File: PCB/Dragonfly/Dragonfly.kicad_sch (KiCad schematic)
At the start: 0 parts

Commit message: hell yeah
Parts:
- added U1: STM32F405RGTx, Package_QFP:LQFP-64_10x10mm_P0.5mm, symbol MCU_ST_STM32F4:STM32F405RGTx
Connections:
- new net: U1.18 (VSS), U1.63 (VSS)
- new net PA0: U1.14 (PA0)
- new net PA1: U1.15 (PA1)
- new net PA10: U1.43 (PA10)
- new net PA11: U1.44 (PA11)
- new net PA12: U1.45 (PA12)
- new net PA13: U1.46 (PA13)
- new net PA14: U1.49 (PA14)
- new net PA15: U1.50 (PA15)
- new net PA2: U1.16 (PA2)
- new net PA3: U1.17 (PA3)
- new net PA4: U1.20 (PA4)
- new net PA5: U1.21 (PA5)
- new net PA6: U1.22 (PA6)
- new net PA7: U1.23 (PA7)
- new net PA8: U1.41 (PA8)
- new net PA9: U1.42 (PA9)
- new net PB0: U1.26 (PB0)
- new net PB1: U1.27 (PB1)
- new net PB10: U1.29 (PB10)
- new net PB11: U1.30 (PB11)
- new net PB12: U1.33 (PB12)
- new net PB13: U1.34 (PB13)
- new net PB14: U1.35 (PB14)
- new net PB15: U1.36 (PB15)
- new net PB2: U1.28 (PB2)
- new net PB3: U1.55 (PB3)
- new net PB4: U1.56 (PB4)
- new net PB5: U1.57 (PB5)
- new net PB6: U1.58 (PB6)
- new net PB7: U1.59 (PB7)
- new net PB8: U1.61 (PB8)
- new net PB9: U1.62 (PB9)
- new net PC0: U1.8 (PC0)
- new net PC1: U1.9 (PC1)
- new net PC10: U1.51 (PC10)
- new net PC11: U1.52 (PC11)
- new net PC12: U1.53 (PC12)
- new net PC13: U1.2 (PC13)
- new net PC14: U1.3 (PC14)
- new net PC15: U1.4 (PC15)
- new net PC2: U1.10 (PC2)
- new net PC3: U1.11 (PC3)
- new net PC4: U1.24 (PC4)
- new net PC5: U1.25 (PC5)
- new net PC6: U1.37 (PC6)
- new net PC8: U1.38 (PC7)
- new net PC9: U1.39 (PC8)

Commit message: updated
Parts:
- added +10ppm: 32.768 kHz, symbol Device:Crystal
- added C1, C2: 100pf, symbol Device:C
- added C3, C4: 12pf, symbol Device:C
- added SW1: SW_SPDT_312, symbol Switch:SW_SPDT_312
- added X1: TSX-3225, TSX-3225, symbol TSX-3225:TSX-3225
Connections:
- net PC9 is gone; now on net PC8: U1.39 (PC8)
- net PC8: no longer U1.38 (PC7)
- net CP9: now reaches U1.40 (PC9)
- net at U1.5 (PH0): now also C1.2, X1.1
- net PD2: now reaches U1.54 (PD2)
- net at U1.6 (PH1): now also C2.2, X1.3
- net BOOT0: now reaches U1.60 (BOOT0)
- net NRST: now reaches U1.7 (NRST)
- net PA14: no longer names the net of U1.49 (PA14)
- net PA14: now also +10ppm.2, C3.1
- net PA15: no longer names the net of U1.50 (PA15)
- net PA15: now also +10ppm.1, C4.1
- new net: C2.1, X1.4
- new net: C1.1, X1.2
- new net GND: C3.2, C4.2
- new net PC7: U1.38 (PC7)
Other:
- note added: "MIAN MCU"
- moved on the sheet: U1

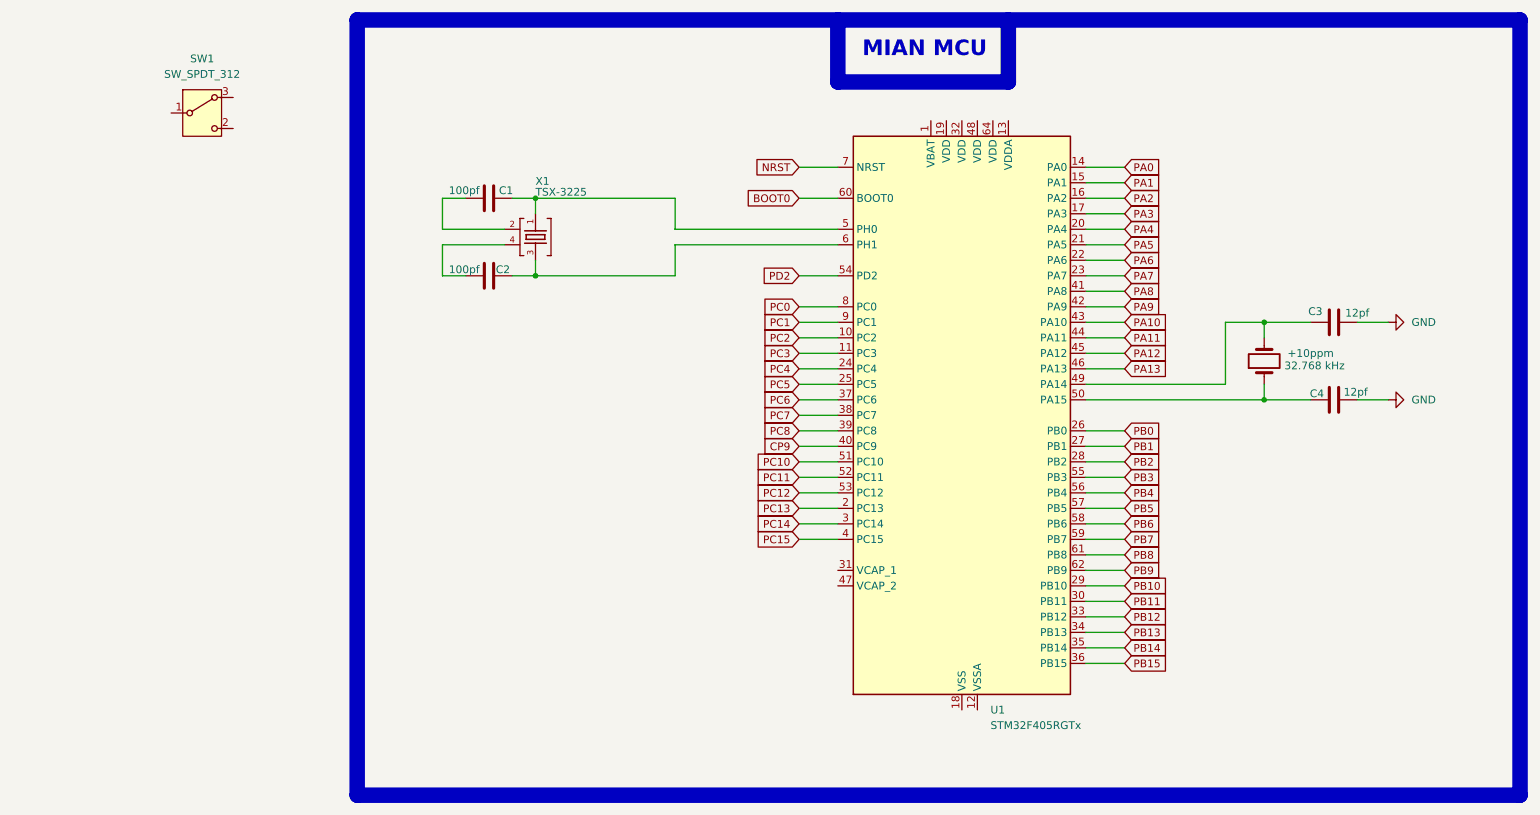
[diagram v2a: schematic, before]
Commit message: updates
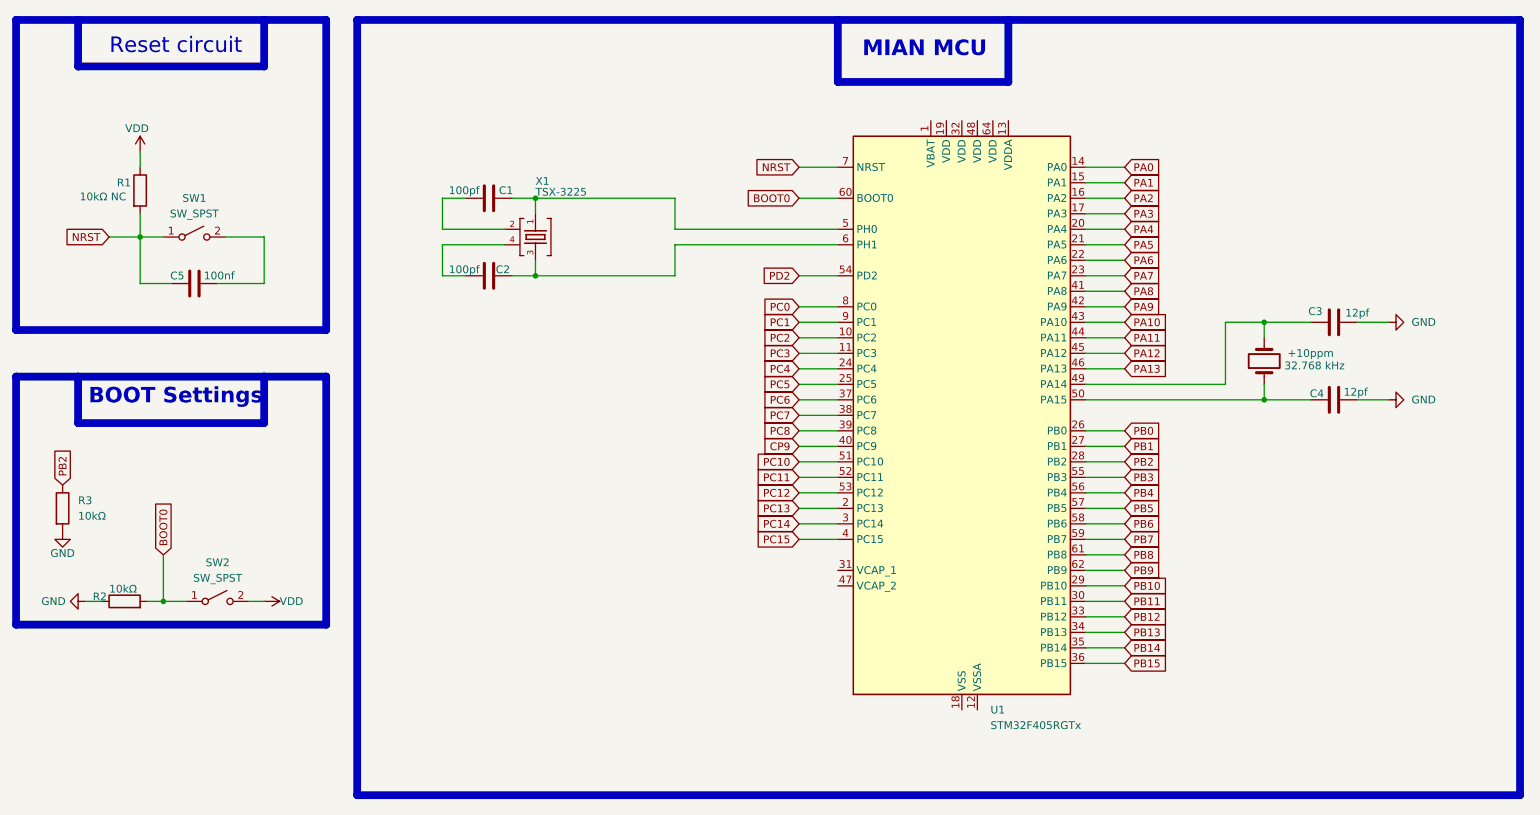
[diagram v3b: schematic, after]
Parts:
- removed SW1: SW_SPDT_312, symbol Switch:SW_SPDT_312
- added C5: 100nf, symbol Device:C
- added R1: 10kΩ NC, symbol Device:R
- added R2, R3: 10kΩ, symbol Device:R
- added SW1, SW2: SW_SPST, symbol Switch:SW_SPST
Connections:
- net BOOT0: now also R2.2, SW2.1 (A)
- net GND: now also R2.1, R3.2
- net NRST: now also C5.1, R1.2, SW1.1 (A)
- net PB2: now also R3.1
- new net: C5.2, SW1.2 (B)
- new net VDD: R1.1, SW2.2 (B)
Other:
- note added: "BOOT Settings"
- note added: "Reset circuit"
